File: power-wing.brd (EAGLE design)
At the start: 50.8 x 22.9 mm, 25 parts, among them T1 2N2222, T2 2N2222, T3 2N2222, U1 TLV2462IP

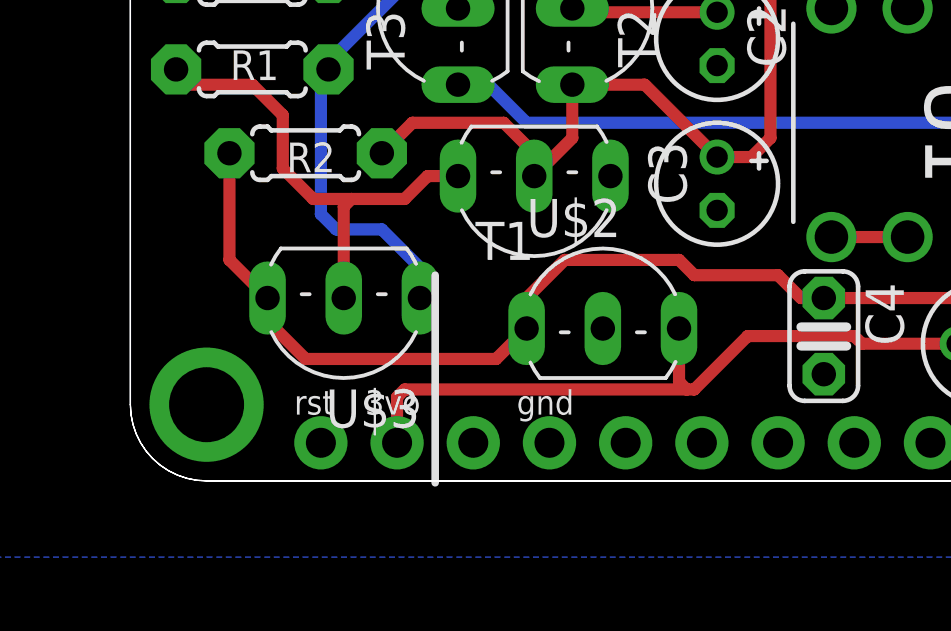
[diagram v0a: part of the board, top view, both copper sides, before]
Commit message: fixed the names
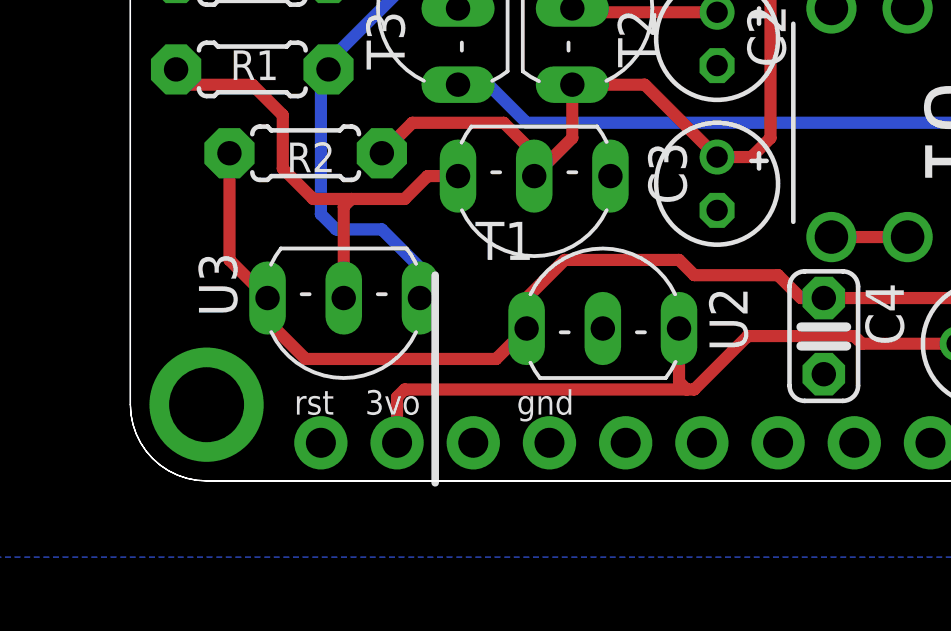
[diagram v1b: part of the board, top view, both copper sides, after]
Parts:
- renumbered U$2 to U2, U$3 to U3
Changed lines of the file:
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@@
 <attribute name="VALUE" x="39.37" y="15.621" size="1.27" layer="27"/>
 </element>
-<element name="U$2" library="dm_parts" package="TO92-BCE" value="L4931" x="15.748" y="5.08"/>
-<element name="U$3" library="dm_parts" package="TO92-BCE" value="VP2206N3-G" x="7.112" y="6.096" rot="R180"/>
+<element name="U2" library="dm_parts" package="TO92-BCE" value="L4931" x="15.748" y="5.08" smashed="yes">
+<attribute name="NAME" x="20.574" y="4.318" size="1.27" layer="25" ratio="10" rot="R90"/>
+<attribute name="VALUE" x="13.208" y="1.778" size="1.27" layer="27" ratio="10"/>
+</element>
+<element name="U3" library="dm_parts" package="TO92-BCE" value="VP2206N3-G" x="7.112" y="6.096" smashed="yes" rot="R180">
+<attribute name="NAME" x="2.286" y="7.62" size="1.27" layer="25" ratio="10" rot="R270"/>
+<attribute name="VALUE" x="9.652" y="9.398" size="1.27" layer="27" ratio="10" rot="R180"/>
+</element>
 </elements>
 <signals>
@@
 <contactref element="C5" pad="-"/>
 <contactref element="R9" pad="1"/>
-<contactref element="U$2" pad="C"/>
+<contactref element="U2" pad="C"/>
 </signal>
 <signal name="AREF">
@@
 <wire x1="24.13" y1="4.826" x2="20.574" y2="4.826" width="0.4064" layer="1"/>
 <wire x1="20.574" y1="4.826" x2="18.796" y2="3.048" width="0.4064" layer="1"/>
-<contactref element="U$2" pad="E"/>
+<contactref element="U2" pad="E"/>
 <wire x1="18.288" y1="5.08" x2="18.288" y2="3.302" width="0.4064" layer="1"/>
 <wire x1="18.288" y1="3.302" x2="18.542" y2="3.048" width="0.4064" layer="1"/>
@@
 <wire x1="4.064" y1="13.208" x2="1.524" y2="13.208" width="0.4064" layer="1"/>
 <wire x1="7.112" y1="9.144" x2="7.366" y2="9.398" width="0.4064" layer="1"/>
-<contactref element="U$3" pad="C"/>
+<contactref element="U3" pad="C"/>
 <wire x1="7.112" y1="6.096" x2="7.112" y2="9.144" width="0.4064" layer="1"/>
 </signal>
@@
 <wire x1="6.35" y1="8.89" x2="6.35" y2="13.462" width="0.4064" layer="16"/>
 <wire x1="6.35" y1="13.462" x2="6.604" y2="13.716" width="0.4064" layer="16"/>
-<contactref element="U$3" pad="B"/>
+<contactref element="U3" pad="B"/>
 <wire x1="9.652" y1="6.096" x2="9.652" y2="7.112" width="0.4064" layer="16"/>
 <wire x1="9.652" y1="7.112" x2="8.382" y2="8.382" width="0.4064" layer="16"/>
@@
 <wire x1="22.352" y1="6.096" x2="23.114" y2="6.096" width="0.4064" layer="1"/>
 <wire x1="3.302" y1="10.922" x2="3.302" y2="7.366" width="0.4064" layer="1"/>
-<contactref element="U$2" pad="B"/>
+<contactref element="U2" pad="B"/>
 <wire x1="5.842" y1="4.064" x2="12.192" y2="4.064" width="0.4064" layer="1"/>
 <wire x1="12.192" y1="4.064" x2="13.208" y2="5.08" width="0.4064" layer="1"/>
@@
 <wire x1="14.478" y1="7.366" x2="18.288" y2="7.366" width="0.4064" layer="1"/>
 <wire x1="18.288" y1="7.366" x2="18.796" y2="6.858" width="0.4064" layer="1"/>
-<contactref element="U$3" pad="E"/>
+<contactref element="U3" pad="E"/>
 <wire x1="4.572" y1="6.096" x2="3.302" y2="7.366" width="0.4064" layer="1"/>
 <wire x1="5.842" y1="4.064" x2="4.572" y2="5.334" width="0.4064" layer="1"/>
